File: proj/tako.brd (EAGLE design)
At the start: 100 x 80 mm, 22 parts, among them U1 ENC28J6028QFN, U2 ARJC02-111008B, X1 25MHz

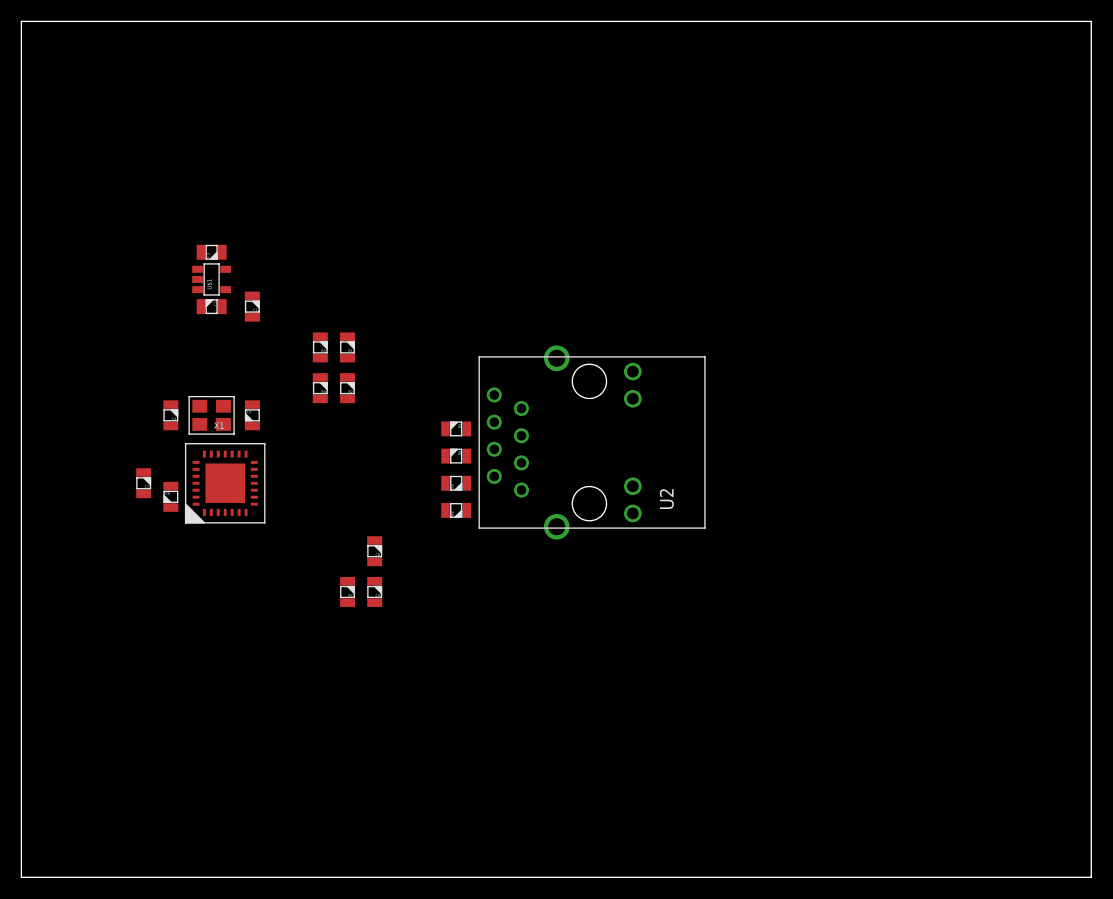
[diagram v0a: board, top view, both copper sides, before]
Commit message: Started designing Tako schematic & board @open #11
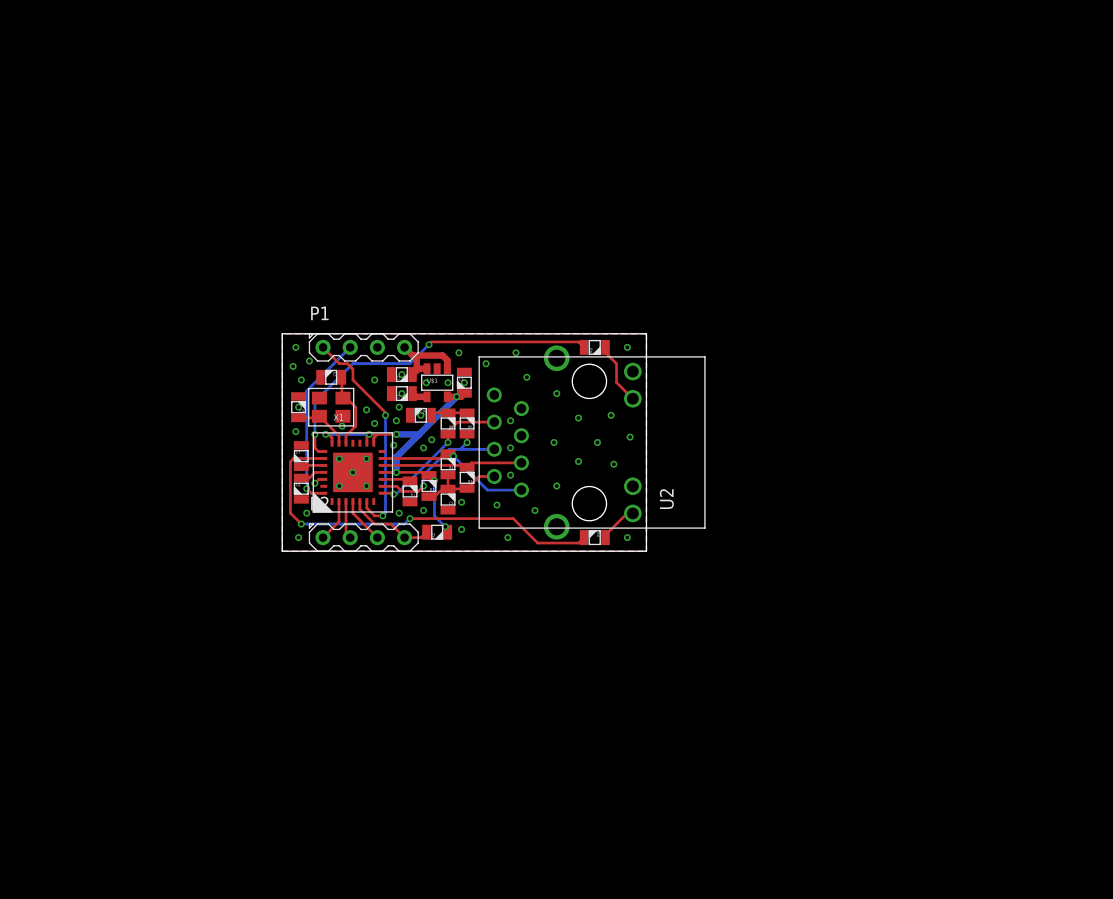
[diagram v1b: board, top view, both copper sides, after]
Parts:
- added P1: RESET-INT-GND-VIN, dooba:PIN_4
- added P2: SO-SI-SCK-CS, dooba:PIN_4
- moved R8 31.2 mm to (53.6, 31.8), turned to 180 degrees
- moved C3 26.6 mm to (41.4, 46.2), turned to 270 degrees
- moved R9 25.9 mm to (53.6, 49.5), turned to 0 degrees
- moved U$1 23.2 mm to (38.9, 46.2), turned to 0 degrees
- moved C2 18.9 mm to (35.6, 47.0), turned to 0 degrees
- moved C1 16.2 mm to (35.6, 45.2), turned to 0 degrees
- moved R2 15.9 mm to (38.9, 32.3), turned to 0 degrees
- moved C7 14.9 mm to (26.2, 39.4), turned to 270 degrees
- moved R1 14.7 mm to (36.3, 36.1)
- moved C8 13.4 mm to (37.3, 43.2), turned to 180 degrees
- moved R7 12.5 mm to (38.1, 36.6)
- moved C6 12.2 mm to (26.2, 36.3)
- moved U1 12.0 mm to (31.0, 37.8)
- moved C4 12.0 mm to (25.9, 43.9)
- moved X1 11.2 mm to (29.0, 43.9)
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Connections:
- removed net N$7: R2.1, U1.5
- new net !WNC28J60_CS: P2.4, R2.1, U1.5
- net !ENC28J60_RESET: now also P1.1
- net ENC28J60_INT: now also P1.2
- net ENC28J60_SCK: now also P2.3
- net ENC28J60_SI: now also P2.2
- net ENC28J60_SO: now also P2.1
- net GND: now also P1.3
- net VIN: now also P1.4
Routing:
- net N$14: track 0.00 -> 37.3 mm, vias 0 -> 2
- net 3.3V: track 0.00 -> 33.5 mm, vias 0 -> 7
- net N$13: track 0.00 -> 33.0 mm, vias 0 -> 2
- net !ENC28J60_RESET: track 0.00 -> 21.1 mm, vias 0 -> 2
- net ENC28J60_INT: track 0.00 -> 16.7 mm, vias 0 -> 1
- net N$11: track 0.00 -> 14.6 mm, vias 0 -> 1
- net N$8: track 0.00 -> 14.6 mm, vias 0 -> 2
- net N$9: track 0.00 -> 13.9 mm, vias 0 -> 2
- net N$10: track 0.00 -> 13.3 mm
- net VIN: track 0.00 -> 8.40 mm
- net !WNC28J60_CS: track 0.00 -> 8.25 mm
- net N$16: track 0.00 -> 8.20 mm
- net N$2: track 0.00 -> 7.27 mm
- net N$17: track 0.00 -> 5.86 mm
- net N$1: track 0.00 -> 5.29 mm
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- added copper zone on layer 1, net GND
- added copper zone on layer 16, net GND
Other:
- board size 100 x 80 mm -> 34 x 20.3 mm
